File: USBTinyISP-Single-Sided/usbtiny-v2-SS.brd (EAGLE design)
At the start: 68.2 x 36.8 mm, 22 parts, among them IC1 ATTINY2313-20P, IC2 74AHC125N, Q1 12Mhz

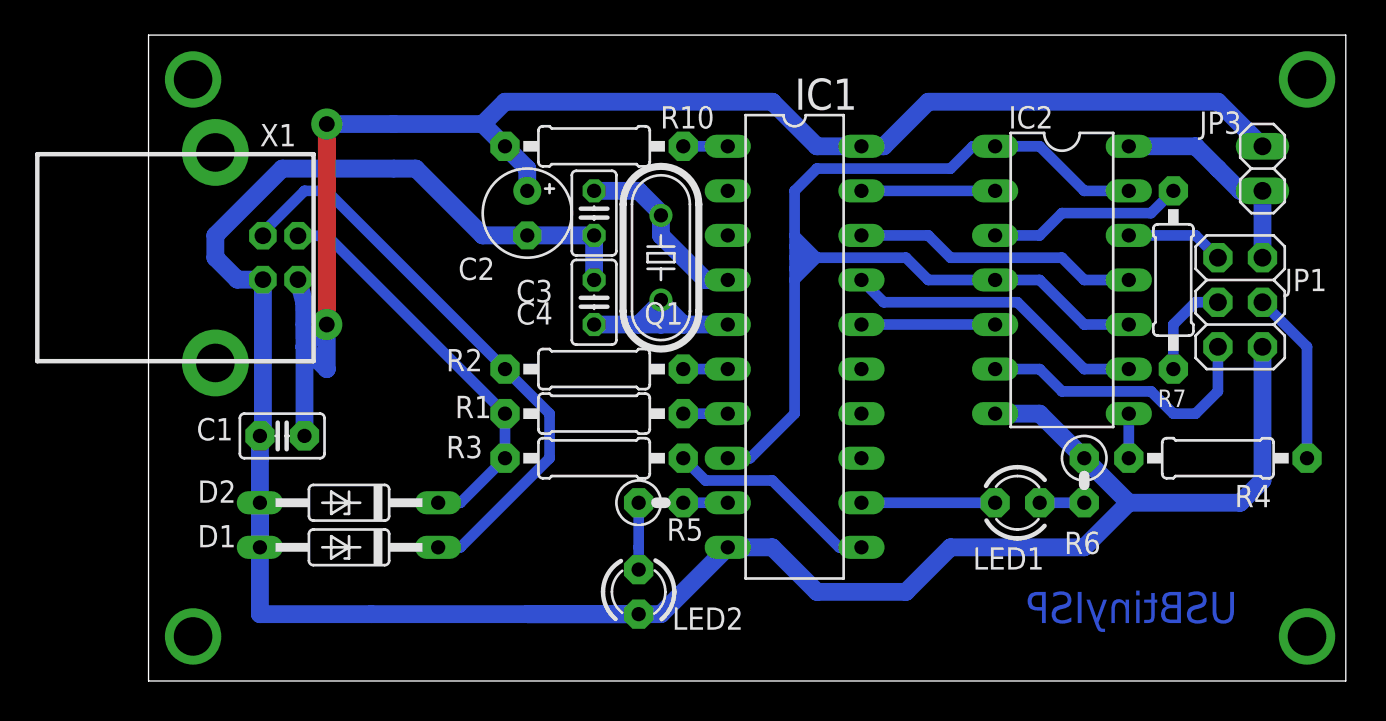
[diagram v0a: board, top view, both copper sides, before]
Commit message: Version 0.05
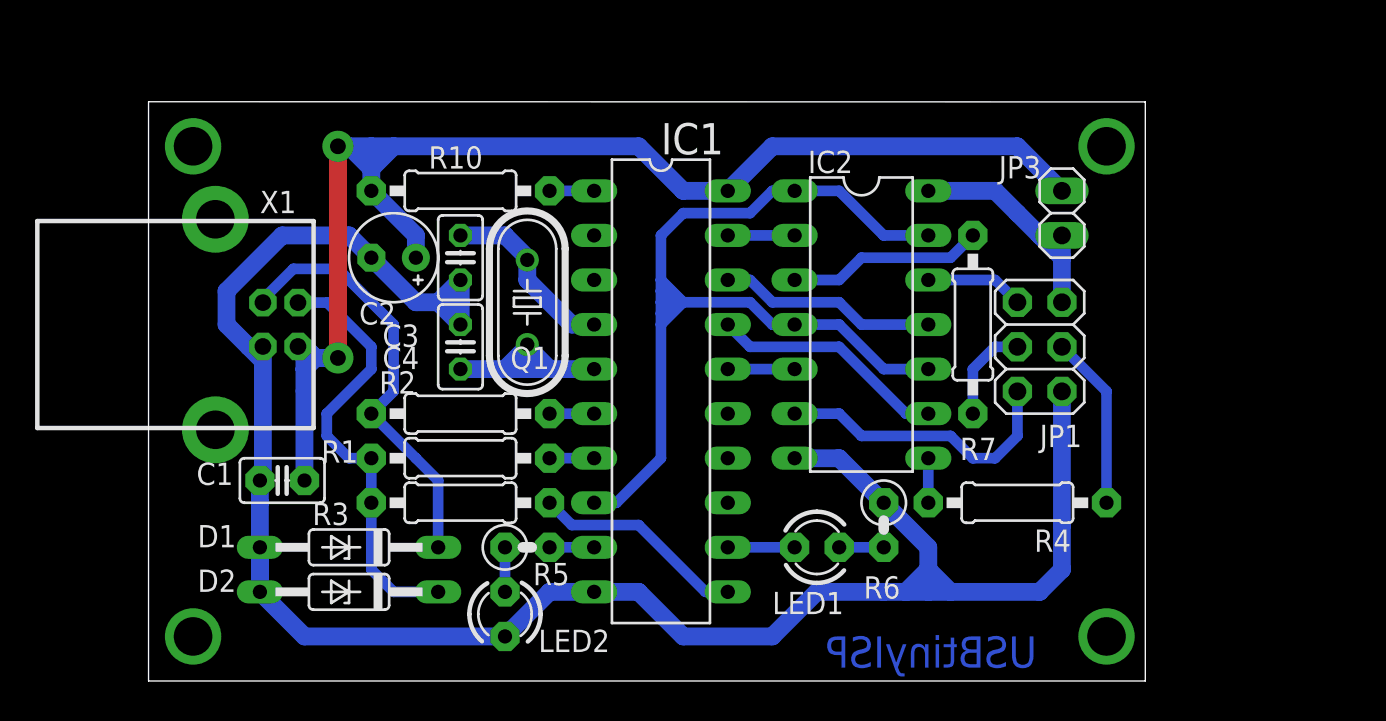
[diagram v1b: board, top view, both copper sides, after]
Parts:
- moved R6 11.7 mm to (41.9, 8.89)
- moved IC2 11.7 mm to (40.6, 20.3)
- moved JP1 11.7 mm to (50.8, 19.1)
- moved JP3 11.7 mm to (52.1, 26.7)
- moved LED1 11.7 mm to (38.1, 7.62)
- moved R4 11.7 mm to (49.5, 10.2)
- moved R7 11.7 mm to (47.0, 20.3)
- moved R5 8.03 mm to (21.6, 7.62)
- moved C2 8.03 mm to (14.0, 24.1), turned to 180 degrees
- moved Q1 8.03 mm to (21.6, 21.6)
- moved C3 8.03 mm to (17.8, 24.1)
- moved C4 8.03 mm to (17.8, 19.1)
- moved IC1 8.03 mm to (29.2, 16.5)
- moved R1 8.03 mm to (17.8, 12.7)
- moved R10 8.03 mm to (17.8, 27.9)
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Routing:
- net GND: track 156.1 -> 135.3 mm
- net N$2: track 33.8 -> 24.5 mm
- net VCC: track 89.7 -> 80.7 mm
- net BUFFEN: track 64.7 -> 57.1 mm
- net MISO': track 16.3 -> 12.5 mm
- net SCK': track 7.62 -> 3.81 mm
- net RST': track 7.62 -> 3.81 mm
- net N$7: track 7.62 -> 3.81 mm
- net MOSI': track 17.3 -> 13.5 mm
- net N$14: track 12.5 -> 14.3 mm
- net N$1: track 23.4 -> 25.1 mm
- net N$11: track 3.81 -> 2.54 mm
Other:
- board size 68.2 x 36.8 mm -> 56.8 x 33 mm
